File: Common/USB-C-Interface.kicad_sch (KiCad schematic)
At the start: 6 parts

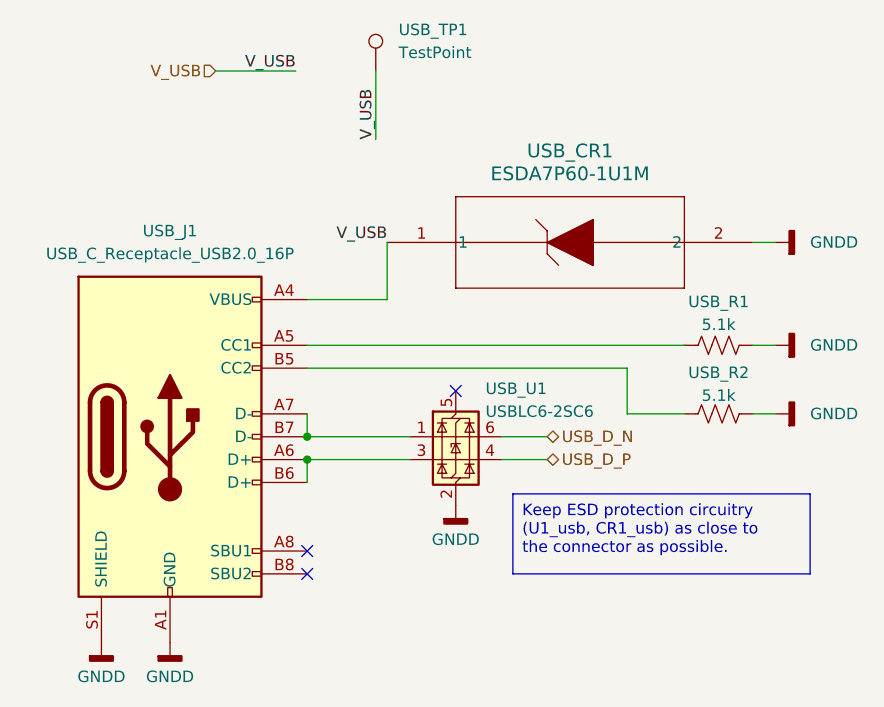
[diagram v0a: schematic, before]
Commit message: Revert "Resolved recovery dev merge"
This reverts commit 81c4bbda93894cf9b120906f02d3dbab6bbd1e60, reversing
changes made to 220360569fc6c62025a0e7a68270d7f77f4a1f37.
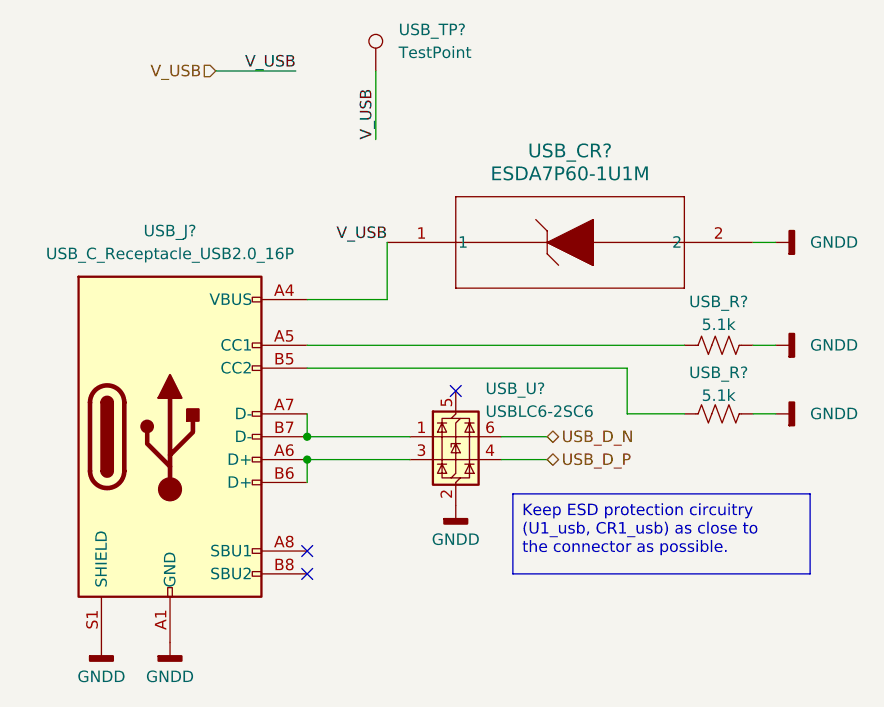
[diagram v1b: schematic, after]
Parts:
- renumbered USB_CR1 to USB_CR?, USB_J1 to USB_J?, USB_R2 to USB_R?, USB_R1 to USB_R?, USB_TP1 to USB_TP?, USB_U1 to USB_U?
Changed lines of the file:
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@@
 		(on_board yes)
 		(dnp no)
-		(property "Reference" "USB_U1"
+		(property "Reference" "USB_U?"
 			(at 82.042 72.136 0)
 			(effects
@@
 		)
 		(instances
-			(project "USB-C-Interface"
-				(path "/7c253a73-a3ad-4431-8c8c-7421e0c0a047"
-					(reference "USB_U1")
-					(unit 1)
-				)
-			)
 			(project "Radio-Module"
 				(path "/acc63f22-7eb8-450a-9af4-da5f4b8157d9/066db7ca-fd8b-46d1-a06b-412eb11482f3"
@@
 		(dnp no)
 		(fields_autoplaced yes)
-		(property "Reference" "USB_J1"
+		(property "Reference" "USB_J?"
 			(at 46.99 54.61 0)
 			(effects
@@
 		)
 		(instances
-			(project "USB-C-Interface"
-				(path "/7c253a73-a3ad-4431-8c8c-7421e0c0a047"
-					(reference "USB_J1")
-					(unit 1)
-				)
-			)
 			(project "Radio-Module"
 				(path "/acc63f22-7eb8-450a-9af4-da5f4b8157d9/066db7ca-fd8b-46d1-a06b-412eb11482f3"
@@
 		(dnp no)
 		(fields_autoplaced yes)
-		(property "Reference" "#PWR02"
+		(property "Reference" "#PWR?"
 			(at 46.99 106.68 0)
 			(effects
@@
 		)
 		(instances
-			(project "USB-C-Interface"
-				(path "/7c253a73-a3ad-4431-8c8c-7421e0c0a047"
-					(reference "#PWR02")
-					(unit 1)
-				)
-			)
 			(project "Radio-Module"
 				(path "/acc63f22-7eb8-450a-9af4-da5f4b8157d9/066db7ca-fd8b-46d1-a06b-412eb11482f3"
@@
 		(dnp no)
 		(fields_autoplaced yes)
-		(property "Reference" "#PWR04"
+		(property "Reference" "#PWR?"
 			(at 120.65 55.88 0)
 			(effects
@@
 		)
 		(instances
-			(project "USB-C-Interface"
-				(path "/7c253a73-a3ad-4431-8c8c-7421e0c0a047"
-					(reference "#PWR04")
-					(unit 1)
-				)
-			)
 			(project "Radio-Module"
 				(path "/acc63f22-7eb8-450a-9af4-da5f4b8157d9/066db7ca-fd8b-46d1-a06b-412eb11482f3"
@@
 		(dnp no)
 		(fields_autoplaced yes)
-		(property "Reference" "#PWR01"
+		(property "Reference" "#PWR?"
 			(at 39.37 106.68 0)
 			(effects
@@
 		)
 		(instances
-			(project "USB-C-Interface"
-				(path "/7c253a73-a3ad-4431-8c8c-7421e0c0a047"
-					(reference "#PWR01")
-					(unit 1)
-				)
-			)
 			(project "Radio-Module"
 				(path "/acc63f22-7eb8-450a-9af4-da5f4b8157d9/066db7ca-fd8b-46d1-a06b-412eb11482f3"
@@
 		(on_board yes)
 		(dnp no)
-		(property "Reference" "USB_R2"
+		(property "Reference" "USB_R?"
 			(at 107.95 70.358 90)
 			(effects
@@
 		)
 		(instances
-			(project "USB-C-Interface"
-				(path "/7c253a73-a3ad-4431-8c8c-7421e0c0a047"
-					(reference "USB_R2")
-					(unit 1)
-				)
-			)
 			(project "Radio-Module"
 				(path "/acc63f22-7eb8-450a-9af4-da5f4b8157d9/066db7ca-fd8b-46d1-a06b-412eb11482f3"
@@
 		(on_board yes)
 		(dnp no)
-		(property "Reference" "USB_R1"
+		(property "Reference" "USB_R?"
 			(at 107.95 62.484 90)
 			(effects
@@
 		)
 		(instances
-			(project "USB-C-Interface"
-				(path "/7c253a73-a3ad-4431-8c8c-7421e0c0a047"
-					(reference "USB_R1")
-					(unit 1)
-				)
-			)
 			(project "Radio-Module"
 				(path "/acc63f22-7eb8-450a-9af4-da5f4b8157d9/066db7ca-fd8b-46d1-a06b-412eb11482f3"
@@
 		(dnp no)
 		(fields_autoplaced yes)
-		(property "Reference" "USB_CR1"
+		(property "Reference" "USB_CR?"
 			(at 91.44 45.72 0)
 			(effects
@@
 		)
 		(instances
-			(project "USB-C-Interface"
-				(path "/7c253a73-a3ad-4431-8c8c-7421e0c0a047"
-					(reference "USB_CR1")
-					(unit 1)
-				)
-			)
 			(project "Radio-Module"
 				(path "/acc63f22-7eb8-450a-9af4-da5f4b8157d9/066db7ca-fd8b-46d1-a06b-412eb11482f3"
@@
 		(dnp no)
 		(fields_autoplaced yes)
-		(property "Reference" "#PWR06"
+		(property "Reference" "#PWR?"
 			(at 120.65 74.93 0)
 			(effects
@@
 		)
 		(instances
-			(project "USB-C-Interface"
-				(path "/7c253a73-a3ad-4431-8c8c-7421e0c0a047"
-					(reference "#PWR06")
-					(unit 1)
-				)
-			)
 			(project "Radio-Module"
 				(path "/acc63f22-7eb8-450a-9af4-da5f4b8157d9/066db7ca-fd8b-46d1-a06b-412eb11482f3"
@@
 		(dnp no)
 		(fields_autoplaced yes)
-		(property "Reference" "#PWR03"
+		(property "Reference" "#PWR?"
 			(at 78.74 91.44 0)
 			(effects
@@
 		)
 		(instances
-			(project "USB-C-Interface"
-				(path "/7c253a73-a3ad-4431-8c8c-7421e0c0a047"
-					(reference "#PWR03")
-					(unit 1)
-				)
-			)
 			(project "Radio-Module"
 				(path "/acc63f22-7eb8-450a-9af4-da5f4b8157d9/066db7ca-fd8b-46d1-a06b-412eb11482f3"
@@
 		(dnp no)
 		(fields_autoplaced yes)
-		(property "Reference" "#PWR05"
+		(property "Reference" "#PWR?"
 			(at 120.65 67.31 0)
 			(effects
@@
 		)
 		(instances
-			(project "USB-C-Interface"
-				(path "/7c253a73-a3ad-4431-8c8c-7421e0c0a047"
-					(reference "#PWR05")
-					(unit 1)
-				)
-			)
 			(project "Radio-Module"
 				(path "/acc63f22-7eb8-450a-9af4-da5f4b8157d9/066db7ca-fd8b-46d1-a06b-412eb11482f3"
@@
 		(dnp no)
 		(fields_autoplaced yes)
-		(property "Reference" "USB_TP1"
+		(property "Reference" "USB_TP?"
 			(at 72.39 32.2579 0)
 			(effects
@@
 		)
 		(instances
-			(project "USB-C-Interface"
-				(path "/7c253a73-a3ad-4431-8c8c-7421e0c0a047"
+			(project "Radio-Module"
+				(path "/acc63f22-7eb8-450a-9af4-da5f4b8157d9/066db7ca-fd8b-46d1-a06b-412eb11482f3"
+					(reference "USB_TP?")
+					(unit 1)
+				)
+			)
+			(project "Main-Module"
+				(path "/c41b490b-5ab6-4438-aea0-388670bb08f4/b23d16a1-3c5b-4321-8b30-5d6992e2f62d"
 					(reference "USB_TP1")
 					(unit 1)
 				)
 			)
-			(project "Radio-Module"
-				(path "/acc63f22-7eb8-450a-9af4-da5f4b8157d9/066db7ca-fd8b-46d1-a06b-412eb11482f3"
-					(reference "USB_TP?")
-					(unit 1)
-				)
-			)
-			(project "Main-Module"
-				(path "/c41b490b-5ab6-4438-aea0-388670bb08f4/b23d16a1-3c5b-4321-8b30-5d6992e2f62d"
-					(reference "USB_TP1")
-					(unit 1)
-				)
-			)
-		)
-	)
-	(sheet_instances
-		(path "/"
-			(page "1")
-		)
-	)
+		)
+	)
